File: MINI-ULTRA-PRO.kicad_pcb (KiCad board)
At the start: 2 copper layers, 25.4 x 55.9 mm, 75 parts, among them J1 S2B-PH-SM4-TB, J2 MICRO-USB, J3 RF-SMA-EDGE_Without_Feed, J4 CONN-HDR-1x19, J5 CONN-HDR-1x19, J6 CONN-HDR-2x5, J7 U.FL-R-SMT, J8 ANTENNA-PAD, M1 MOUNT_HOLE, M2 MOUNT_HOLE, M3 MOUNT_HOLE, M4 MOUNT_HOLE, M5 FIDUCIAL, M6 FIDUCIAL, Q1 2N7002LT1G, SW1 SPNO, U1 ATSAMD21G18A-AU, U2 BQ24074RGTT, U3 RFM95W, U4 MCP1700T-3302E/MB, U5 W25Q16JVSSIM, U6 24AA02E64T-I/OT, Y1 FC-135

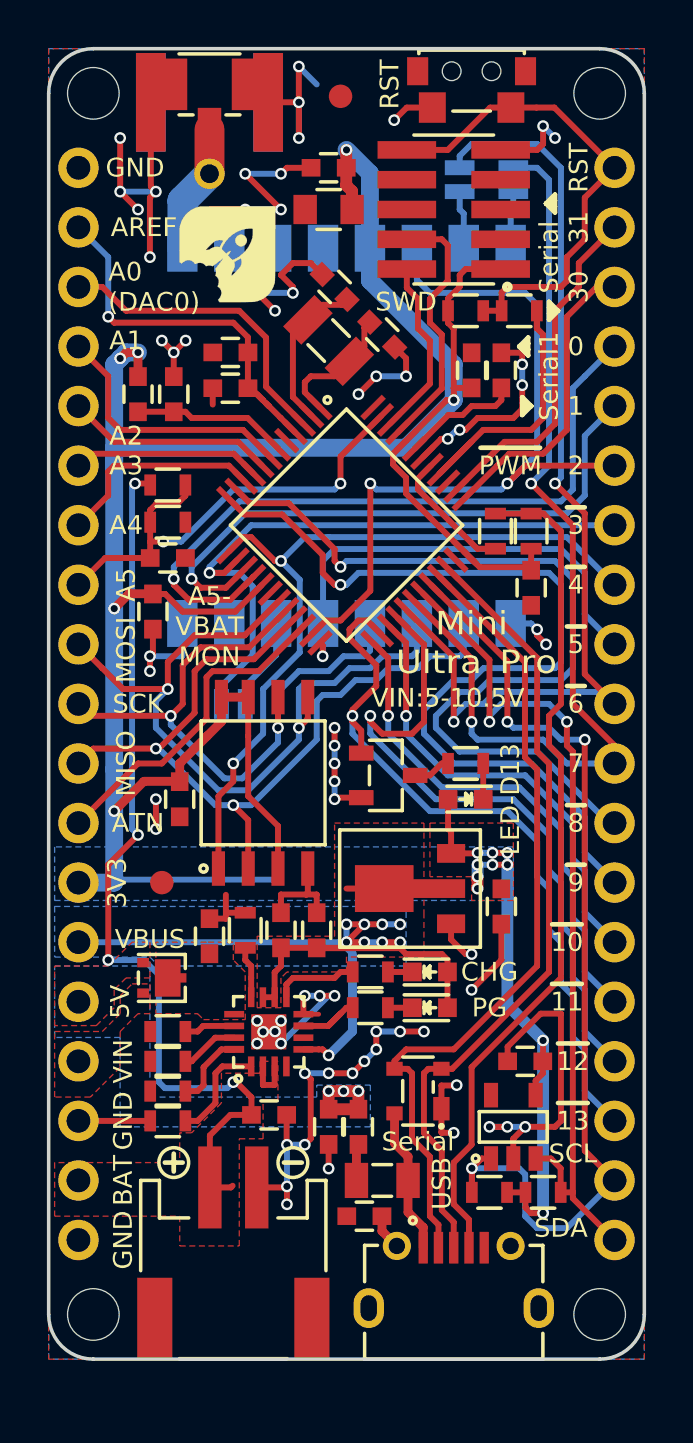
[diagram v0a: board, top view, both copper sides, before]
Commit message: Version 4.00 - V4
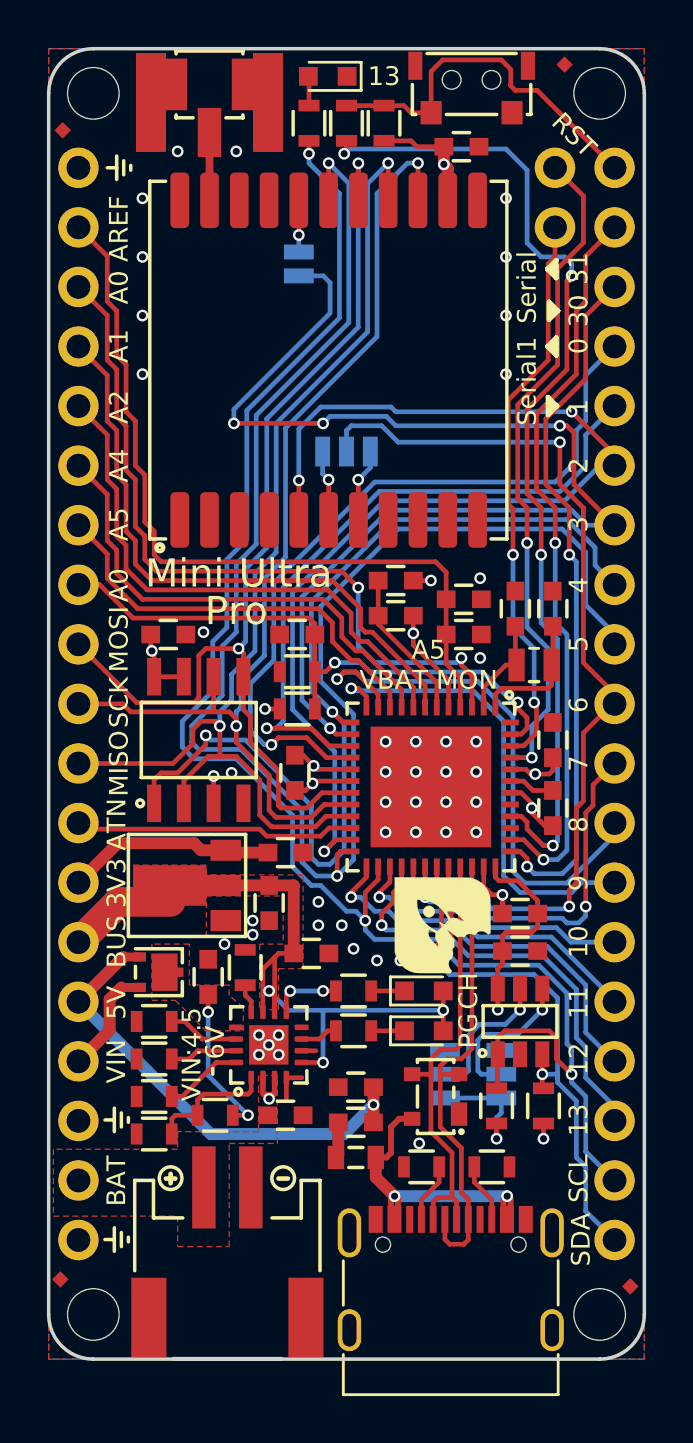
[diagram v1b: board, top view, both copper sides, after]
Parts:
- removed the C12 at (138.9, 76.2)
- removed the C15 at (138.4, 108.7)
- removed the C4 at (132.3, 85.9)
- removed the D1 at (144.8, 103.1)
- removed the J6 at (144.3, 78.0)
- removed J8: ANTENNA-PAD, RocketScreamKicadLibrary:ANTENNA-PAD
- removed the L1 at (140.2, 117.1)
- removed L3: BLM18KG221SN1D, RocketScreamKicadLibrary:I_0603
- removed Q1: 2N7002LT1G, RocketScreamKicadLibrary:SOT-23
- removed the R8 at (132.1, 116.8)
- removed the U1 at (139.7, 91.4)
- added C14: 100nF, RocketScreamKiCadLib:C_0603, F.Cu at (141.8, 95.3)
- added C7: 1uF 50V X5R, RocketScreamKiCadLib:C_0603, F.Cu at (133.8, 110.7)
- added D5: Yellow, RocketScreamKiCadLib:LED_0603, F.Cu at (138.9, 72.3)
- added J3: CONN-HDR-1x2, RocketScreamKiCadLib:HDR_1x2_Pitch2.54mm_WithoutSilk, F.Cu at (148.6, 77.5)
- added JP3: JUMPER-2-WAY, RocketScreamKiCadLib:JUMPER-2-WAY-SMD, B.Cu at (139.7, 88.3)
- added L2: BLM18KG221SN1D, RocketScreamKiCadLib:I_0603, F.Cu at (140.1, 116.9)
- added M7: FIDUCIAL, RocketScreamKiCadLib:FIDUCIAL-0.5MM_SQUARE, F.Cu at (127.5, 123.6)
- added M8: FIDUCIAL, RocketScreamKiCadLib:FIDUCIAL-0.5MM_SQUARE, F.Cu at (151.8, 123.9)
- added R11: 49K9, RocketScreamKiCadLib:R_0603, F.Cu at (131.5, 117.4)
- added R12: 200K, RocketScreamKiCadLib:R_0603, F.Cu at (134.1, 116.6)
- added U4: W25Q16JVSNIM, RocketScreamKiCadLib:SOIC-8-N_8S1, F.Cu at (133.4, 100.6)
- C1, C2: value 18pF -> 10pF; footprint RocketScreamKicadLibrary:C_0603 -> RocketScreamKiCadLib:C_0603
- C10: renamed from C19; value 1uF 10V X5R -> 10uF 16V X5R; footprint RocketScreamKicadLibrary:C_0603 -> RocketScreamKiCadLib:C_0603
- C11: renamed from C14; value 4.7uF 10V X5R -> 10uF 16V X5R; footprint RocketScreamKicadLibrary:C_0603 -> RocketScreamKiCadLib:C_0603
- C12: renamed from C6; footprint RocketScreamKicadLibrary:C_0603 -> RocketScreamKiCadLib:C_0603
- C13: renamed from C18; footprint RocketScreamKicadLibrary:C_0603 -> RocketScreamKiCadLib:C_0603
- C15: renamed from C16; value 4.7uF 10V X5R -> 10uF 16V X5R; footprint RocketScreamKicadLibrary:C_0603 -> RocketScreamKiCadLib:C_0603
- C16: renamed from C13; footprint RocketScreamKicadLibrary:C_0603 -> RocketScreamKiCadLib:C_0603
- C17: renamed from C10; value 4.7uF 10V X5R -> 10uF 16V X5R; footprint RocketScreamKicadLibrary:C_0603 -> RocketScreamKiCadLib:C_0603
- C18: renamed from C20; footprint RocketScreamKicadLibrary:C_0603 -> RocketScreamKiCadLib:C_0603
- C19: renamed from C11; value 47uF 10V X5R -> 22uF 10V X5R; footprint RocketScreamKicadLibrary:C_0805 -> RocketScreamKiCadLib:C_0603
- C3: footprint RocketScreamKicadLibrary:C_0603 -> RocketScreamKiCadLib:C_0603
- C4: renamed from C5; value 1uF 10V X5R -> 1uF 50V X5R; footprint RocketScreamKicadLibrary:C_0603 -> RocketScreamKiCadLib:C_0603
- C5: renamed from C7; footprint RocketScreamKicadLibrary:C_0603 -> RocketScreamKiCadLib:C_0603
- C6: renamed from C8; footprint RocketScreamKicadLibrary:C_0603 -> RocketScreamKiCadLib:C_0603
- C8: renamed from C17; value 4.7uF 10V X5R -> 10uF 16V X5R; footprint RocketScreamKicadLibrary:C_0603 -> RocketScreamKiCadLib:C_0603
- C9: value 1uF 50V X5R -> 10uF 16V X5R; footprint RocketScreamKicadLibrary:C_0603 -> RocketScreamKiCadLib:C_0603
- D1: renamed from D2; footprint RocketScreamKicadLibrary:LED_0603 -> RocketScreamKiCadLib:LED_0603
- D2: renamed from D3; footprint RocketScreamKicadLibrary:LED_0603 -> RocketScreamKiCadLib:LED_0603
- D3: renamed from D4; footprint RocketScreamKicadLibrary:SOT-1016 -> RocketScreamKiCadLib:SOT-1016
- D4: renamed from D5; footprint RocketScreamKicadLibrary:SOT-143B -> RocketScreamKiCadLib:SOT-143B
- F1: value MF-PSMF050X-2 -> MF-FSMF050X-2; footprint RocketScreamKicadLibrary:MF-PSMF020X -> RocketScreamKiCadLib:MF-FSMF
- J1: footprint RocketScreamKicadLibrary:S2B-PH-SM4-TB -> RocketScreamKiCadLib:S2B-PH-SM4-TB
- J2: value MICRO-USB -> USB-C_16Pins; footprint RocketScreamKicadLibrary:MICRO-USB -> RocketScreamKiCadLib:USB-TYPE-C-16PIN-SMD
- J4: renamed from J7; footprint RocketScreamKicadLibrary:U.FL-R-SMT_Extended -> RocketScreamKiCadLib:U.FL-R-SMT_Extended
- J5: renamed from J3; footprint RocketScreamKicadLibrary:RF-SMA-EDGE_Without_Feed -> RocketScreamKiCadLib:RF-SMA-EDGE_Without_Feed
- J6: renamed from J4; footprint RocketScreamKicadLibrary:HDR_1x19_Pitch2.54mm_WithoutSilk -> RocketScreamKiCadLib:HDR_1x19_Pitch2.54mm_WithoutSilk
- J7: renamed from J5; footprint RocketScreamKicadLibrary:HDR_1x19_Pitch2.54mm_WithoutSilk -> RocketScreamKiCadLib:HDR_1x19_Pitch2.54mm_WithoutSilk
- JP1, JP2: value JUMPER-1-WAY -> JUMPER-2-WAY; footprint RocketScreamKicadLibrary:JUMPER-1-WAY-SMD -> RocketScreamKiCadLib:JUMPER-2-WAY-SMD
- JP4: renamed from JP3; footprint RocketScreamKicadLibrary:JUMPER-1-WAY-SMD -> RocketScreamKiCadLib:JUMPER-1-WAY-SMD
- L1: renamed from L2; footprint RocketScreamKicadLibrary:I_0603 -> RocketScreamKiCadLib:I_0603
- LOGO1: footprint RocketScreamKicadLibrary:LOGO-ROCKET-SCREAM_Vertical_Small -> RocketScreamKiCadLib:LOGO-ROCKET-SCREAM_Vertical_Small
- LOGO2: renamed from LOGO4; footprint RocketScreamKicadLibrary:LOGO-ROCKET-SCREAM_Without_Text_XXXSmall -> RocketScreamKiCadLib:LOGO-ROCKET-SCREAM_Without_Text_XXXSmall
- LOGO3: footprint RocketScreamKicadLibrary:LOGO-KICAD_XSmall -> RocketScreamKiCadLib:LOGO-KICAD_XSmall
- LOGO4: renamed from LOGO2; footprint RocketScreamKicadLibrary:LOGO-OSHW_Small -> RocketScreamKiCadLib:LOGO-OSHW_Small
- M1, M2, M3, M4: footprint RocketScreamKicadLibrary:HOLE_NPTH_2.2MM -> RocketScreamKiCadLib:HOLE_NPTH_2.2MM
- M5, M6: footprint RocketScreamKicadLibrary:FIDUCIAL-1MM -> RocketScreamKiCadLib:FIDUCIAL-0.5MM_SQUARE
- R1: renamed from R4; footprint RocketScreamKicadLibrary:R_0603 -> RocketScreamKiCadLib:R_0603
- R10, R2: footprint RocketScreamKicadLibrary:R_0603 -> RocketScreamKiCadLib:R_0603
- R13: renamed from R1; value 2K2 -> 5K1; footprint RocketScreamKicadLibrary:R_0603 -> RocketScreamKiCadLib:R_0603
- R14: renamed from R11; value 100K -> 5K1; footprint RocketScreamKicadLibrary:R_0603 -> RocketScreamKiCadLib:R_0603
- R15: renamed from R3; value 330R -> 5K1; footprint RocketScreamKicadLibrary:R_0603 -> RocketScreamKiCadLib:R_0603
- R16: renamed from R14; footprint RocketScreamKicadLibrary:R_0603 -> RocketScreamKiCadLib:R_0603
- R17: renamed from R5; footprint RocketScreamKicadLibrary:R_0603 -> RocketScreamKiCadLib:R_0603
- R3: renamed from R12; value 2K2 -> 5K1; footprint RocketScreamKicadLibrary:R_0603 -> RocketScreamKiCadLib:R_0603
- R4: renamed from R13; value 2K2 -> 5K1; footprint RocketScreamKicadLibrary:R_0603 -> RocketScreamKiCadLib:R_0603
- R5: renamed from R15; footprint RocketScreamKicadLibrary:R_0603 -> RocketScreamKiCadLib:R_0603
- R6: renamed from R16; footprint RocketScreamKicadLibrary:R_0603 -> RocketScreamKiCadLib:R_0603
- R7: renamed from R6; footprint RocketScreamKicadLibrary:R_0603 -> RocketScreamKiCadLib:R_0603
- R8: renamed from R7; footprint RocketScreamKicadLibrary:R_0603 -> RocketScreamKiCadLib:R_0603
- R9: value 2K94 -> 0R; footprint RocketScreamKicadLibrary:R_0603 -> RocketScreamKiCadLib:R_0603
- SW1: footprint RocketScreamKicadLibrary:TS-018 -> RocketScreamKiCadLib:TS-1086E-12
- U1: renamed from U4; value MCP1700T-3302E/MB -> ME6210A33PG; footprint RocketScreamKicadLibrary:SOT-89 -> RocketScreamKiCadLib:SOT-89_Microchip
- U2: value BQ24074RGTT -> BQ24075T; footprint RocketScreamKicadLibrary:QFN-16_3x3mm -> RocketScreamKiCadLib:QFN-16_3x3mm_TI
- U3: value RFM95W -> ATSAMD21G18A-MU; footprint RocketScreamKicadLibrary:RFM9xW -> RocketScreamKiCadLib:QFN-48-1EP_7x7mm_Pitch0.5mm; moved to F.Cu
- U5: value W25Q16JVSSIM -> 24AA025E64T-I-OT; footprint RocketScreamKicadLibrary:SOIC-8-W -> RocketScreamKiCadLib:SOT-23-6
- U6: value 24AA02E64T-I/OT -> E19-900M20S2; footprint RocketScreamKicadLibrary:SOT-23-5 -> RocketScreamKiCadLib:E19-900M20S2
- Y1: value FC-135 -> FC-12M; footprint RocketScreamKicadLibrary:ABS07 -> RocketScreamKiCadLib:SC-20S
- moved JP2 38.3 mm to (143.9, 114.8), turned to 90 degrees
- moved JP1 38.2 mm to (146.3, 114.8), turned to 90 degrees
- moved U6 33.6 mm to (138.9, 84.4)
- moved M5 32.4 mm to (127.6, 74.6)
- moved LOGO2 30.1 mm to (143.8, 108.5), turned to 90 degrees
- moved R13 28.1 mm to (138.1, 74.3), turned to 90 degrees
- moved R14 27.5 mm to (142.9, 118.8), turned to 180 degrees
- moved R15 27.1 mm to (145.9, 118.8), turned to 0 degrees
- moved JP4 19.0 mm to (137.7, 80.3), turned to -90 degrees
- moved C4 18.8 mm to (148.5, 103.5), turned to -90 degrees
- moved Y1 16.4 mm to (147.7, 97.4), turned to 0 degrees
- moved C3 16.1 mm to (148.5, 100.6)
- moved C1 15.7 mm to (146.9, 95.0), turned to -90 degrees
- moved U3 15.4 mm to (143.3, 102.6), turned to -90 degrees
- moved U5 15.0 mm to (147.1, 112.6), turned to 0 degrees
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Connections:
- C4 pad 1: Net-(C5-Pad1) -> Net-(C4-Pad1)
- C9 pad 1: GND -> VBUS
- C9 pad 2: VEXT -> GND
- J1 pad 3: Net-(J1-Pad3) -> unconnected-(J1-Pad3)
- J1 pad 4: Net-(J1-Pad4) -> unconnected-(J1-Pad4)
- J2 pad 1: VUSB -> GND
- J2 pad 2: /USB- -> GND
- J2 pad 3: /USB+ -> GND
- J2 pad 4: Net-(J2-Pad4) -> GND
- J4 pad 1: Net-(J7-Pad1) -> Net-(J4-Pad1)
- JP1 pad 1: /D6 -> 3V3
- JP2 pad 1: /D7 -> 3V3
- JP4 pad 1: Net-(JP3-Pad1) -> Net-(JP4-Pad1)
- L1 pad 1: Net-(C4-Pad1) -> Net-(C14-Pad1)
- R13 pad 1: Net-(D1-Pad1) (its old number) -> /D13
- R14 pad 1: Net-(J2-Pad4) -> Net-(J2-PadA5)
- R14 pad 2: 3V3 -> GND
- R15 pad 1: Net-(J2-Pad4) -> Net-(J2-PadB5)
- R15 pad 2: /USB_ID -> GND
- SW1 pad 1: GND -> /RST
- SW1 pad 2: /RST -> GND
- U3 pad 1: GND -> Net-(C2-Pad2)
- U3 pad 10: GND -> /A4
- U3 pad 11: Net-(U3-Pad11) -> /D8
- U3 pad 12: Net-(U3-Pad12) -> /D9
- U3 pad 13: 3V3 -> /D4
- U3 pad 14: /D2 -> /D3
- U3 pad 15: Net-(JP1-Pad2) -> /D1
- U3 pad 16: Net-(JP2-Pad2) -> /D0
- U3 pad 2: /MISO -> Net-(C1-Pad2)
- U3 pad 3: /MOSI -> /A0
- U3 pad 4: /SCK -> AREF
- U3 pad 5: /D5 -> GND
- U3 pad 6: Net-(JP3-Pad1) -> Net-(C14-Pad1)
- U3 pad 7: Net-(U3-Pad7) -> /A1
- U3 pad 8: GND -> /A2
- U3 pad 9: Net-(J7-Pad1) -> /A3
- U5 pad 1: /D4 -> /SCL
- U5 pad 2: /MISO -> GND
- U5 pad 3: 3V3 -> /SDA
- U5 pad 4: GND -> Net-(JP1-Pad2)
- U5 pad 5: /MOSI -> Net-(JP2-Pad2)
- U5 pad 6: /SCK -> 3V3
- U6 pad 1: /SCL -> GND
- U6 pad 3: /SDA -> GND
- U6 pad 4: 3V3 -> GND
- U6 pad 5: Net-(U6-Pad5) -> /D2
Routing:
- net 3V3: track 154.6 -> 38.3 mm, vias 16 -> 9
- net GND: track 122.4 -> 17.9 mm, vias 68 -> 49
- net /D5: track 20.3 -> 71.0 mm, vias 1 -> 2
- net Net-(J2-Pad4): track 36.2 -> 0.00 mm
- net /RESET: track 12.5 -> 42.9 mm, vias 0 -> 4
- net /D13: track 31.9 -> 60.6 mm, vias 1 -> 2
- net /D7: track 41.7 -> 15.7 mm
- net /D3: track 27.3 -> 51.0 mm, vias 1 -> 4
- net VBAT: track 41.4 -> 20.6 mm, vias 4 -> 2
- net /D9: track 39.7 -> 20.1 mm
- net /A0: track 13.2 -> 32.0 mm, vias 0 -> 2
- net /SCK: track 27.8 -> 45.9 mm
- net AREF: track 16.2 -> 34.1 mm, vias 1 -> 0
- net /SWCLK: track 11.1 -> 28.5 mm, vias 0 -> 2
- net /SCL: track 42.2 -> 25.2 mm, vias 3 -> 2
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- added copper zone on In2.Cu, net 3V3
- added copper zone on In1.Cu, net GND
- removed copper zone on B.Cu, net 3V3
- removed copper zone on F.Cu, net 3V3
- removed copper zone on B.Cu, net 5V0
- removed copper zone on F.Cu, net 5V0
- removed copper zone on B.Cu, net VBUS
- removed copper zone on F.Cu, net VIN
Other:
- copper layers 2 -> 4
- net class Default removed
- net class RF-50Ohm removed
- rule pad_to_mask_clearance: 0.1016 -> 0.04
- board text added: "433MHz"
- board text added: "4V00 2022-06"
- board text added: "6V"
- board text added: "868/915MHz"
- board text added: "A0"
- board text added: "A5 VBAT MON"
- board text added: "BQ24074"
- board text added: "BQ24075T"
- board text added: "BUS"
- board text added: "CH"
- board text added: "EUI I2C ADD"
- board text added: "H"
- board text added: "L"
- board text added: "LMIC"
- board text added: "SWCLK"
- board text added: "SWDIO"
- board text added: "VIN:4.5"
- board text removed: "433MHZ"
- board text removed: "868MHZ"
- board text removed: "915MHZ"
- board text removed: "A0 (DAC0)"
- board text removed: "A3"
- board text removed: "A5- VBAT MON"
- board text removed: "CHG"
- board text removed: "D3"
- board text removed: "D6"
- board text removed: "D7"
- board text removed: "EUI64:"
- board text removed: "GND"
- board text removed: "LED-D13"
- board text removed: "Mini Ultra Pro 01-2018 0v50"
- board text removed: "PWM"
- board text removed: "RFM69"
- board text removed: "RFM95"
- board text removed: "RFM95T"
- board text removed: "SWD"
- board text removed: "USB"
- board text removed: "VBUS"
- board text removed: "VIN:5-10.5V"
